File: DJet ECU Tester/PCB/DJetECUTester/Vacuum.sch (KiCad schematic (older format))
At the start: 13 parts, among them J7 VAC, Q10 MMBT2222ALT1G, Q9 MMBT2222ALT1G

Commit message: Working on ECU tester and ECU outputs board.
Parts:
- J7: footprint (none) -> TerminalBlock_TE-Connectivity:TerminalBlock_TE_282834-5_1x05_P2.54mm_Horizontal; manf# (none) -> 282834-5
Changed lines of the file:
@@
 $Descr A4 11693 8268
 encoding utf-8
-Sheet 6 6
+Sheet 6 7
 Title "D-Jetronic ECU Tester"
-Date "2021-03-04"
+Date "2021-03-08"
 Rev "1.0"
 Comp "(C) Britishideas 2021"
@@
 F 0 "J7" H 7930 3442 50  0000 L CNN
 F 1 "VAC" H 7930 3351 50  0000 L CNN
-F 2 "" H 7850 3400 50  0001 C CNN
+F 2 "TerminalBlock_TE-Connectivity:TerminalBlock_TE_282834-5_1x05_P2.54mm_Horizontal" H 7850 3400 50  0001 C CNN
 F 3 "~" H 7850 3400 50  0001 C CNN
+F 4 "282834-5" H 7850 3400 50  0001 C CNN "manf#"
 	1    7850 3400
 	1    0    0    -1

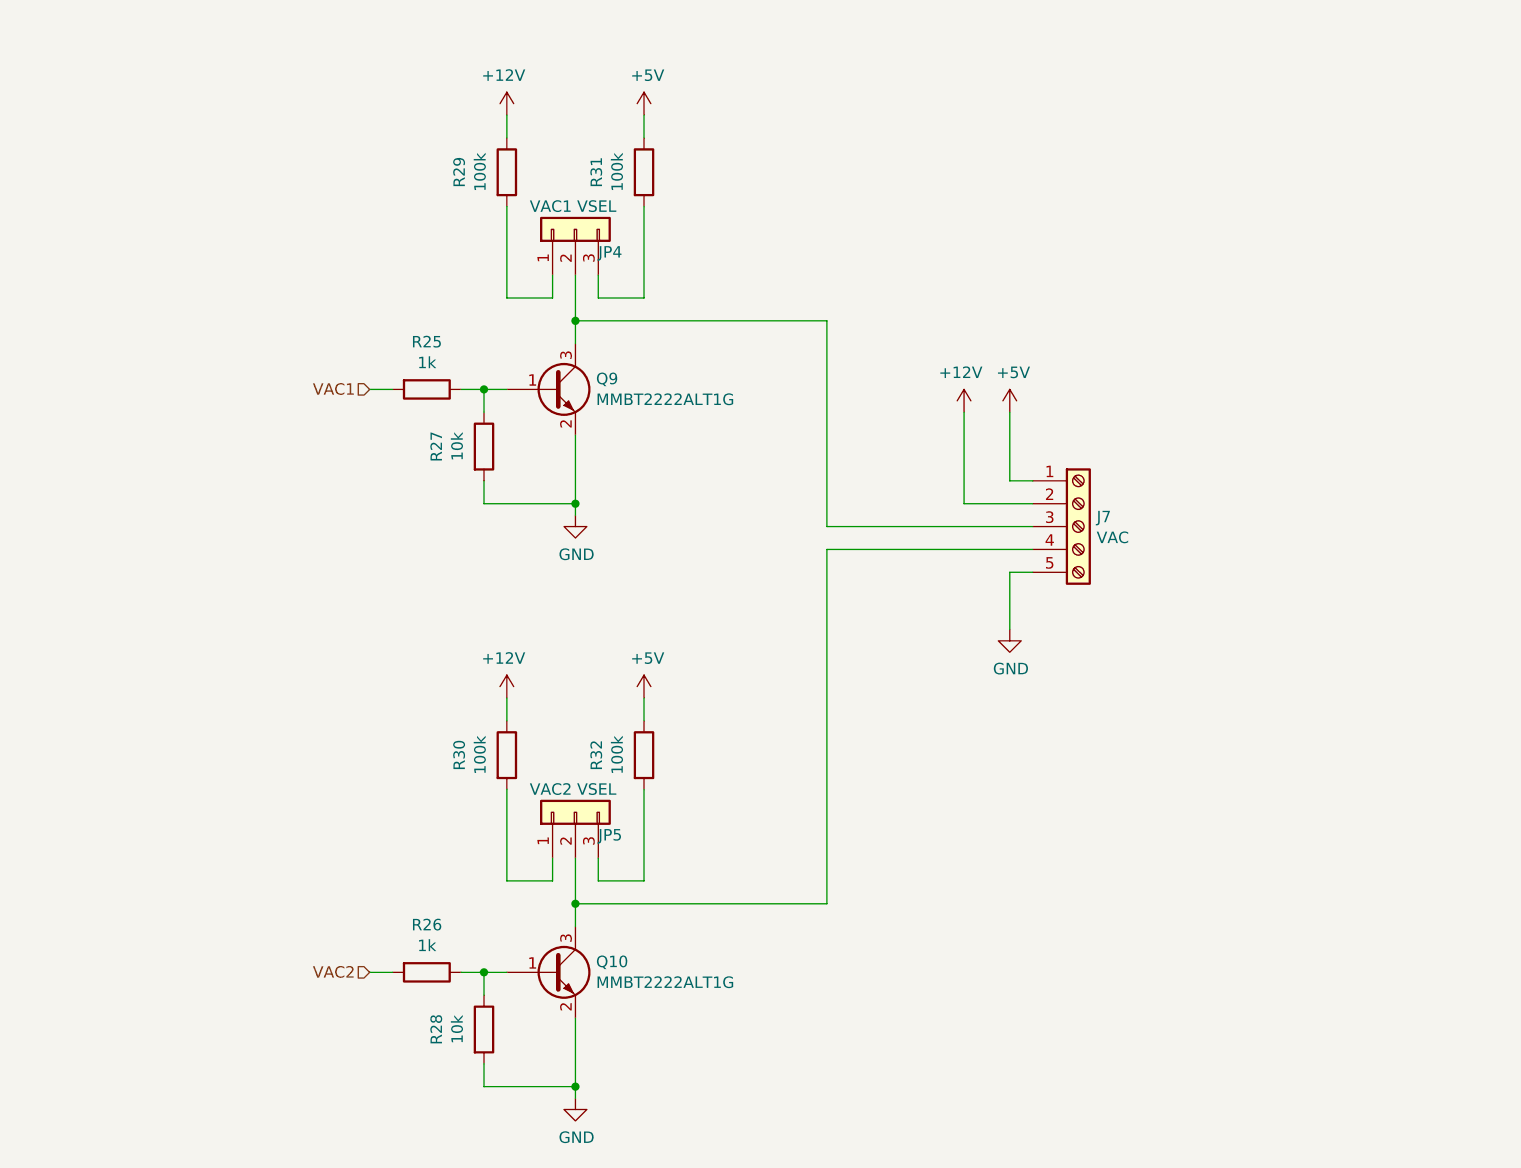
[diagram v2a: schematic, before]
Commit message: Working on PCB layout
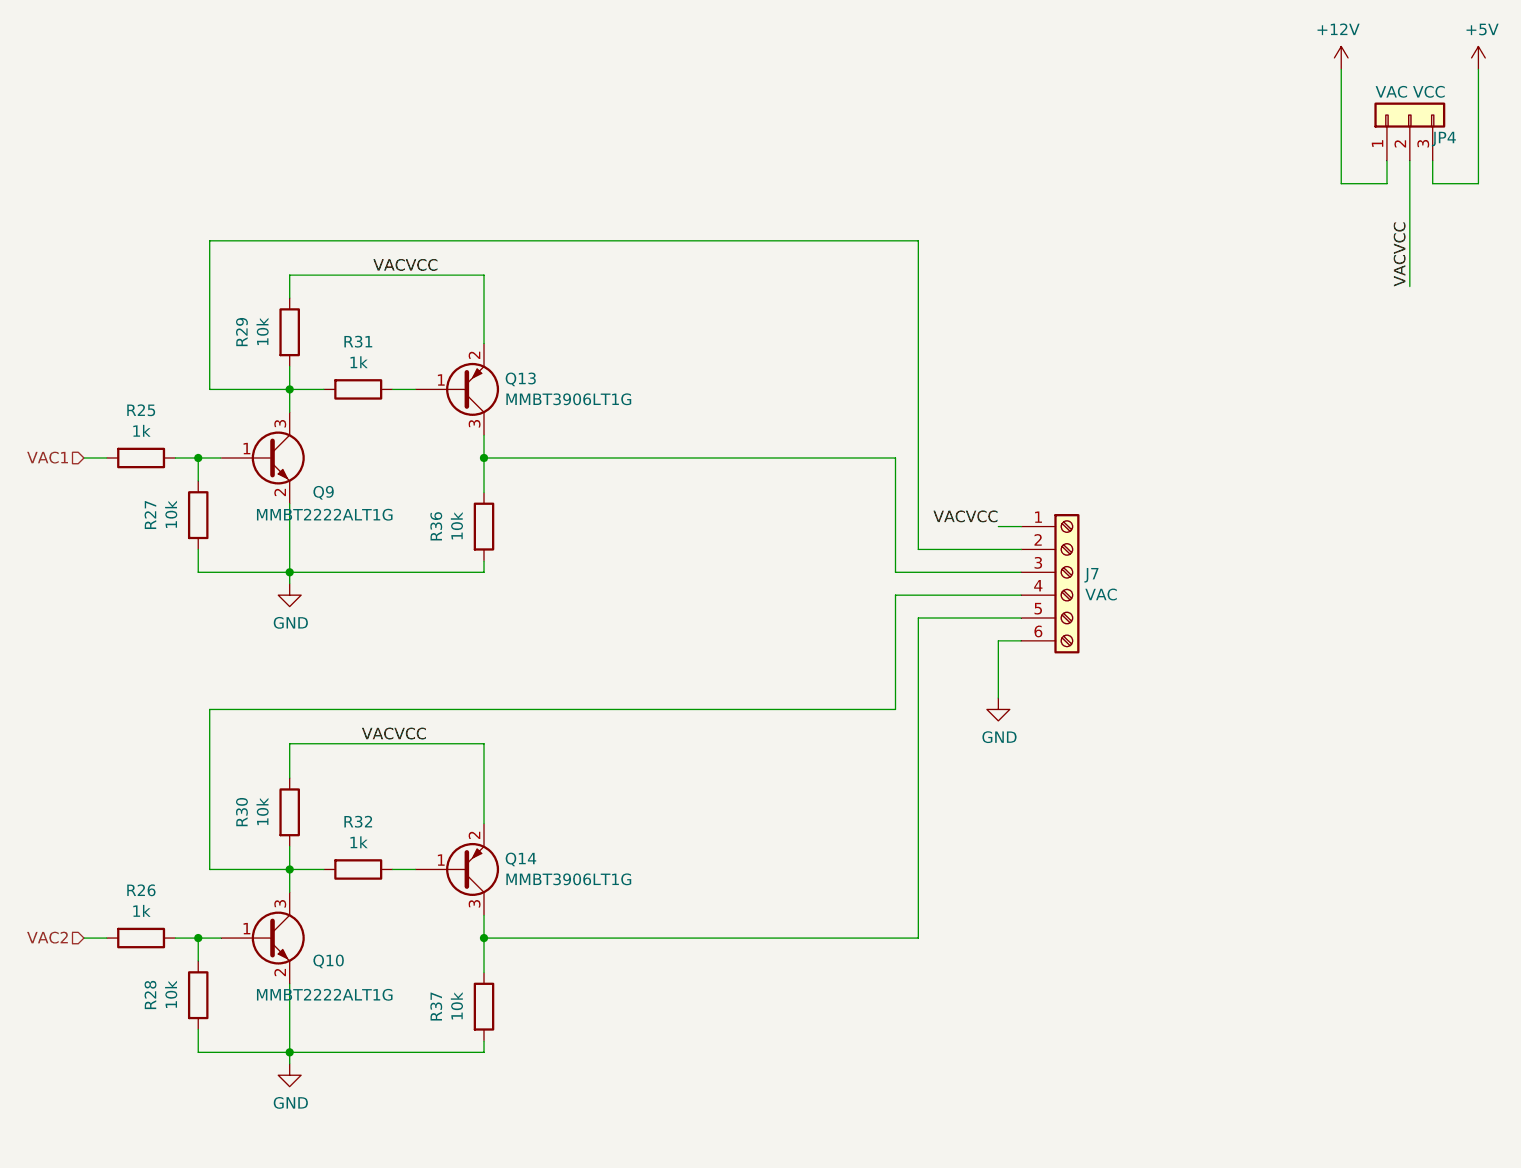
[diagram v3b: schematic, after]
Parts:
- removed J7: VAC, TerminalBlock_TE-Connectivity:TerminalBlock_TE_282834-5_1x05_P2.54mm_Horizontal, symbol Connector:Screw_Terminal_01x05
- removed JP5: VAC2 VSEL, Connector_PinHeader_2.54mm:PinHeader_1x03_P2.54mm_Vertical, symbol Connector_Generic:Conn_01x03
- added J7: VAC, TerminalBlock_TE-Connectivity:TerminalBlock_TE_282834-6_1x06_P2.54mm_Horizontal, symbol Connector:Screw_Terminal_01x06
- added Q13, Q14: MMBT3906LT1G, Package_TO_SOT_SMD:SOT-23, symbol Device:Q_PNP_BEC
- added R36, R37: 10k, Resistor_SMD:R_0805_2012Metric, symbol Device:R
- JP4: value VAC1 VSEL -> VAC VCC
- R29, R30: value 100k -> 10k
- R31, R32: value 100k -> 1k
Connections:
- net +12V: now also JP4.1 (Pin_1); no longer R29.1, R30.1
- net +5V: now also JP4.3 (Pin_3); no longer R31.1, R32.1
- net GND: now also J7.6 (Pin_6), R36.2, R37.2
- net at Q9.3 (C): now also R29.2, R31.2, J7.2 (Pin_2); no longer JP4.2 (Pin_2)
- net at Q10.3 (C): now also R30.2, R32.2, J7.4 (Pin_4)
- new net: Q13.1 (B), R31.1
- new net: J7.3 (Pin_3), Q13.3 (C), R36.1
- new net: J7.5 (Pin_5), Q14.3 (C), R37.1
- new net: Q14.1 (B), R32.1
- new net VACVCC: J7.1 (Pin_1), JP4.2 (Pin_2), Q13.2 (E), Q14.2 (E), R29.1, R30.1
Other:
- moved on the sheet: JP4, Q10, Q9, R25, R26, R27, R28

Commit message: Updated manufacturer part numbers. Working on ECU outputs tester board.
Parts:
- J7: manf# (none) -> 282834-6
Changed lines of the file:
@@
 F 2 "TerminalBlock_TE-Connectivity:TerminalBlock_TE_282834-6_1x06_P2.54mm_Horizontal" H 7800 3600 50  0001 C CNN
 F 3 "~" H 7800 3600 50  0001 C CNN
+F 4 "282834-6" H 7800 3600 50  0001 C CNN "manf#"
 	1    7800 3600
 	1    0    0    -1
